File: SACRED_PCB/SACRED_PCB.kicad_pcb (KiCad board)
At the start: 2 copper layers, 134.7 x 78 mm, 43 parts, among them J1 Screw_Terminal_01x02, J10 Conn_01x14, J11 Conn_01x13, J12 Screw_Terminal_01x04, J13 Screw_Terminal_01x02, J14 Conn_01x16, J2 Analog 0, J3 Analog 1, J4 Stepper 0, J5 Stepper 1, J6 Analog 2, J7 Stepper 2, J8 Stepper 3, J9 Analog 3, U1 AMS1117-5.0, U2 AMS1117-3.3, U3 Teensy4.1, U4 CD74HCT4067QM96Q, U5 OPA607Q1

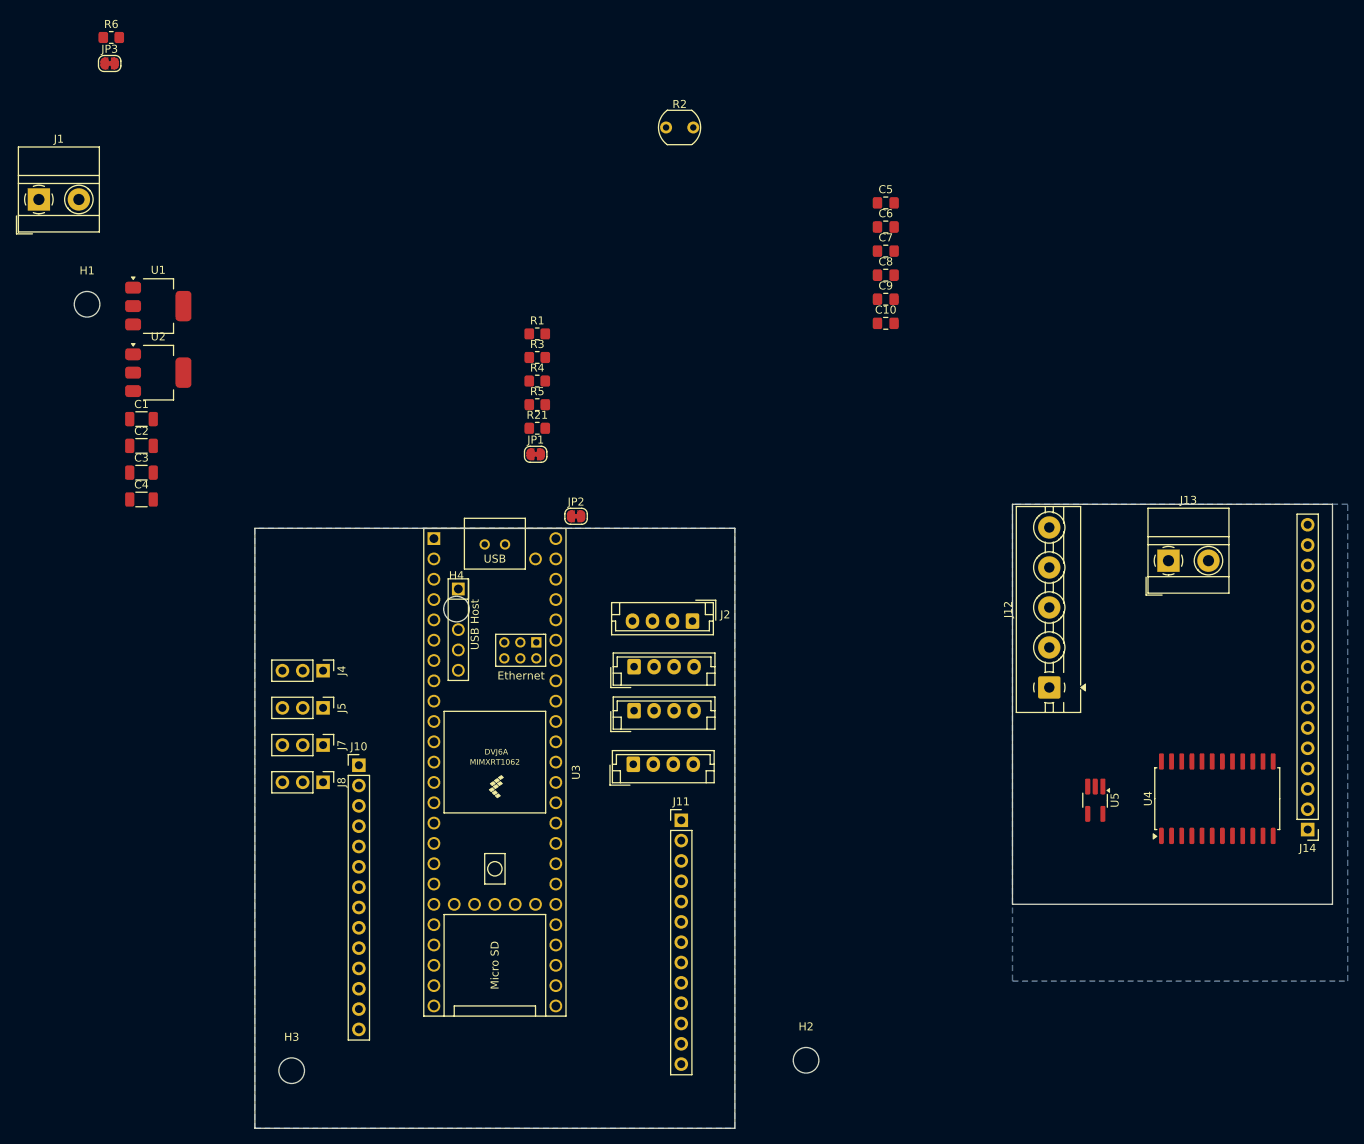
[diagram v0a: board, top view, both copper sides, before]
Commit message: PCB Rev 0.1
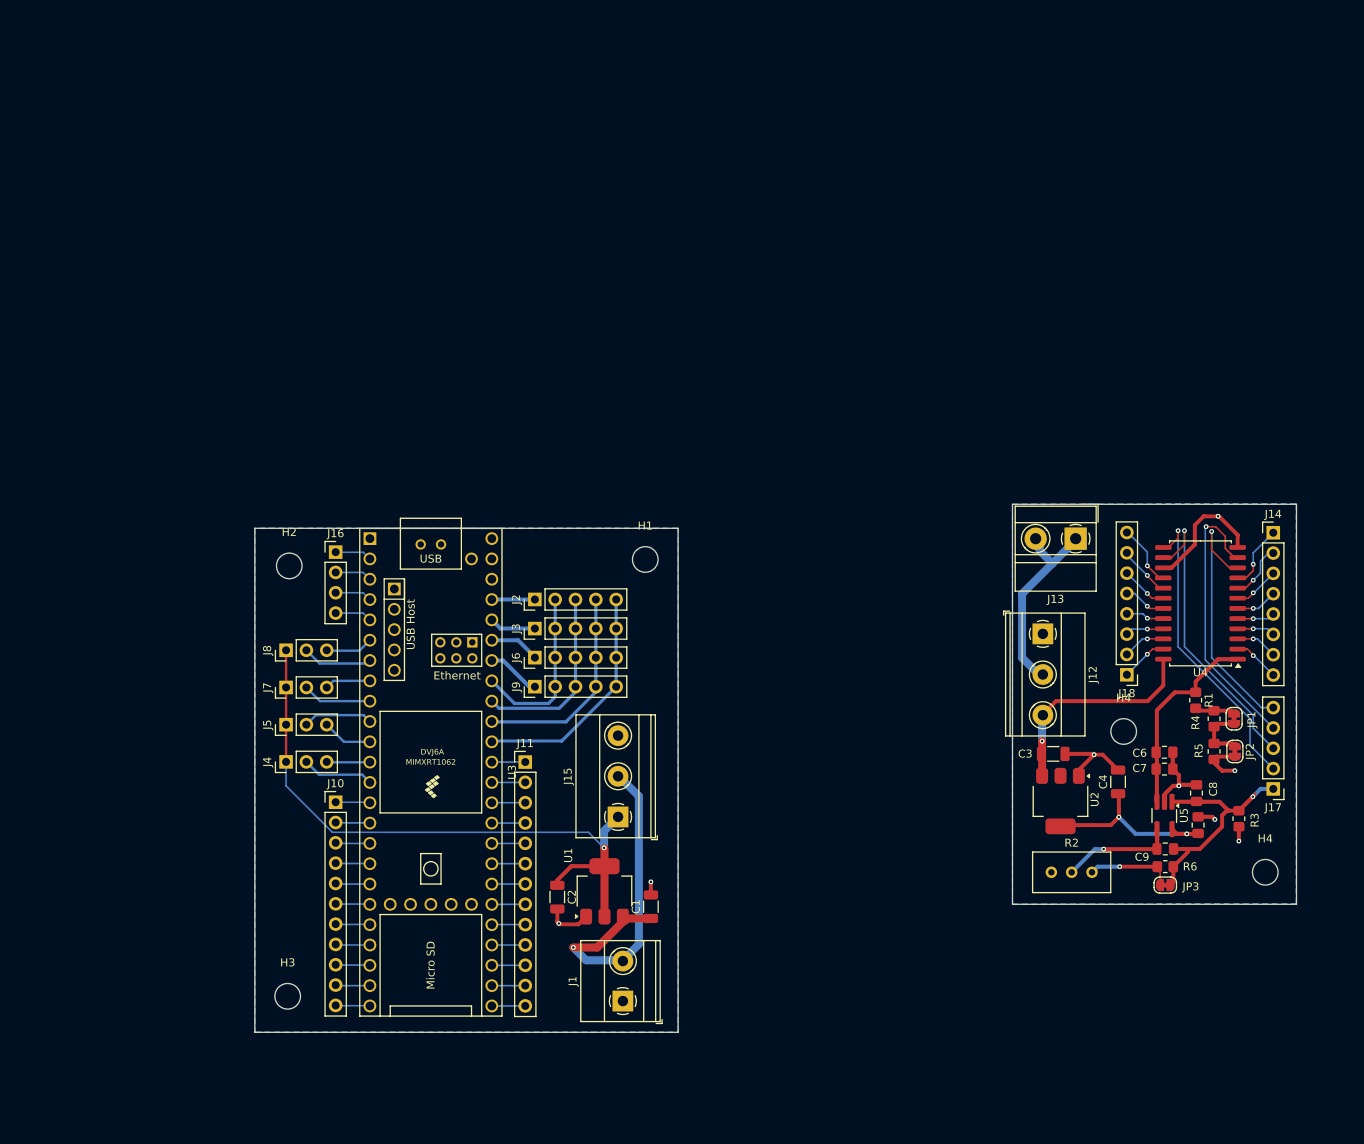
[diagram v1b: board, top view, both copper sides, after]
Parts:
- removed C10: 100nF, Capacitor_SMD:C_0805_2012Metric_Pad1.18x1.45mm_HandSolder
- removed R21: 3M, Resistor_SMD:R_0805_2012Metric_Pad1.20x1.40mm_HandSolder
- added H4: MountingHole, MountingHole:MountingHole_3.2mm_M3, F.Cu at (206.4, 119.1)
- added J15: Screw_Terminal_01x04, TerminalBlock_Phoenix:TerminalBlock_Phoenix_MKDS-1,5-3-5.08_1x03_P5.08mm_Horizontal, F.Cu at (143.2, 129.8)
- added J16: Conn_01x04, Connector_PinHeader_2.54mm:PinHeader_1x04_P2.54mm_Vertical, F.Cu at (107.9, 96.7)
- added J17: Analog 0, Connector_PinHeader_2.54mm:PinHeader_1x05_P2.54mm_Vertical, F.Cu at (225.1, 126.3)
- added J18: Conn_01x16, Connector_PinHeader_2.54mm:PinHeader_1x08_P2.54mm_Vertical, F.Cu at (206.8, 112.0)
- J1: footprint TerminalBlock_MetzConnect:TerminalBlock_MetzConnect_Type011_RT05502HBWC_1x02_P5.00mm_Horizontal -> TerminalBlock_Phoenix:TerminalBlock_Phoenix_MKDS-1,5-2_1x02_P5.00mm_Horizontal
- J10: value Conn_01x14 -> Conn_01x11; footprint Connector_PinHeader_2.54mm:PinHeader_1x14_P2.54mm_Vertical -> Connector_PinHeader_2.54mm:PinHeader_1x11_P2.54mm_Vertical
- J12: footprint TerminalBlock:TerminalBlock_MaiXu_MX126-5.0-05P_1x05_P5.00mm -> TerminalBlock_Phoenix:TerminalBlock_Phoenix_MKDS-1,5-3-5.08_1x03_P5.08mm_Horizontal
- J14: footprint Connector_PinHeader_2.54mm:PinHeader_1x16_P2.54mm_Vertical -> Connector_PinHeader_2.54mm:PinHeader_1x08_P2.54mm_Vertical
- J2, J3, J6, J9: footprint Connector_JST:JST_EH_B4B-EH-A_1x04_P2.50mm_Vertical -> Connector_PinHeader_2.54mm:PinHeader_1x05_P2.54mm_Vertical
- R2: footprint OptoDevice:R_LDR_5.1x4.3mm_P3.4mm_Vertical -> Potentiometer_THT:Potentiometer_Bourns_3296W_Vertical
- moved R6 167.6 mm to (211.6, 136.0), turned to 180 degrees
- moved JP3 167.2 mm to (211.6, 138.3), turned to 180 degrees
- moved C4 127.1 mm to (205.7, 125.4), turned to 90 degrees
- moved U2 124.8 mm to (198.5, 127.8), turned to -90 degrees
- moved J1 124.0 mm to (143.8, 152.8), turned to 90 degrees
- moved C3 119.3 mm to (197.6, 121.9)
- moved R2 107.2 mm to (202.4, 136.7)
- moved H4 106.3 mm to (224.1, 136.7)
- moved R3 105.0 mm to (220.8, 130.0), turned to 90 degrees
- moved R5 95.1 mm to (217.7, 121.6), turned to -90 degrees
- moved R4 94.5 mm to (217.7, 117.5), turned to -90 degrees
- moved R1 94.2 mm to (215.4, 115.2), turned to -90 degrees
- moved JP1 93.3 mm to (220.2, 117.5), turned to 90 degrees
- moved U1 92.0 mm to (141.5, 139.1), turned to 90 degrees
- moved H2 89.4 mm to (102.1, 98.4)
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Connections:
- J1 pad 1: +12V -> GND
- J1 pad 2: GND -> +12V
- J10 pad 1: /Pin_0 -> /Pin_12
- J10 pad 10: /Pin_28 -> /Pin_31
- J10 pad 11: /Pin_29 -> /Pin_32
- J10 pad 2: /Pin_1 -> /Pin_3v3
- J10 pad 3: /Pin_2 -> /Pin_24
- J10 pad 4: /Pin_3 -> /Pin_25
- J10 pad 5: /Pin_3v3 -> /Pin_26
- J10 pad 6: /Pin_24 -> /Pin_27
- J10 pad 7: /Pin_25 -> /Pin_28
- J10 pad 8: /Pin_26 -> /Pin_29
- J10 pad 9: /Pin_27 -> /Pin_30
- J12 pad 1: +12V -> GND
- J12 pad 2: +5V -> +12V
- J12 pad 3: +3.3V -> +5V
- J4 pad 1: /Stepper_EN -> +5V
- J5 pad 1: /Stepper_EN -> +5V
- J7 pad 1: /Stepper_EN -> +5V
- J8 pad 1: /Stepper_EN -> +5V
- U3 pad 11: /Stepper_2_STEP -> /Stepper_1_DIR
- U3 pad 12: /Stepper_2_DIR -> /Stepper_0_STEP
- U3 pad 13: /Stepper_3_STEP -> /Stepper_0_DIR
- U3 pad 14: /Stepper_3_DIR -> /Pin_12
- U3 pad 6: /Stepper_EN -> /Stepper_3_DIR
- U3 pad 7: /Stepper_0_DIR -> /Stepper_3_STEP
- U3 pad 8: /Stepper_0_STEP -> /Stepper_2_DIR
- U3 pad 9: /Stepper_1_DIR -> /Stepper_2_STEP
- U4 pad 16: Net-(J14-Pin_16) -> Net-(J18-Pin_8)
- U4 pad 17: Net-(J14-Pin_15) -> Net-(J18-Pin_7)
- U4 pad 18: Net-(J14-Pin_14) -> Net-(J18-Pin_6)
- U4 pad 19: Net-(J14-Pin_13) -> Net-(J18-Pin_5)
- U4 pad 20: Net-(J14-Pin_12) -> Net-(J18-Pin_4)
- U4 pad 21: Net-(J14-Pin_11) -> Net-(J18-Pin_3)
- U4 pad 22: Net-(J14-Pin_10) -> Net-(J18-Pin_2)
- U4 pad 23: Net-(J14-Pin_9) -> Net-(J18-Pin_1)
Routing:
- net +5V: track 0.00 -> 108.6 mm, vias 0 -> 2
- net +12V: track 0.00 -> 70.0 mm, vias 0 -> 1
- net /MUX_3: track 0.00 -> 67.3 mm, vias 0 -> 1
- net /MUX_2: track 0.00 -> 63.0 mm, vias 0 -> 1
- net /MUX_1: track 0.00 -> 58.8 mm, vias 0 -> 1
- net /MUX_0: track 0.00 -> 54.8 mm, vias 0 -> 1
- net GND: track 0.00 -> 54.7 mm, vias 0 -> 8
- net /Analog_0: track 0.00 -> 35.0 mm, vias 0 -> 1
- net Net-(U4-COM): track 0.00 -> 25.0 mm
- net +3.3V: track 0.00 -> 23.6 mm, vias 0 -> 2
- net Net-(U5--): track 0.00 -> 14.4 mm, vias 0 -> 1
- net Net-(JP3-B): track 0.00 -> 10.9 mm, vias 0 -> 1
- net /Stepper_0_DIR: track 0.00 -> 9.00 mm
- net /Stepper_3_STEP: track 0.00 -> 8.78 mm
- net /Stepper_1_STEP: track 0.00 -> 8.77 mm
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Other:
- board size 134.7 x 78 mm -> 130.2 x 66 mm
